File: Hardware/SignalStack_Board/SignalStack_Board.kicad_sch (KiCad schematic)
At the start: 66 parts, among them J1 Molex_uF_SV_06, J2 RJ45_LED_Shielded, J3 Molex_uF_SV_06, Q1 SI4156DY, Q2 SI4156DY, Q3 SI4156DY, Q4 SI4156DY, Q5 SI4156DY, Q6 SI4156DY, Q7 SI4156DY, Q8 SI4156DY, U1 OKI, U10 74LVC2G04, U2 SMAJ12CA, U3 Teensy4.1_DEV-16771, U4 TSR_1-2450, U5 IRS2005S, U6 IRS2005S, U7 74LVC2G04, U8 IRS2005S, U9 IRS2005S

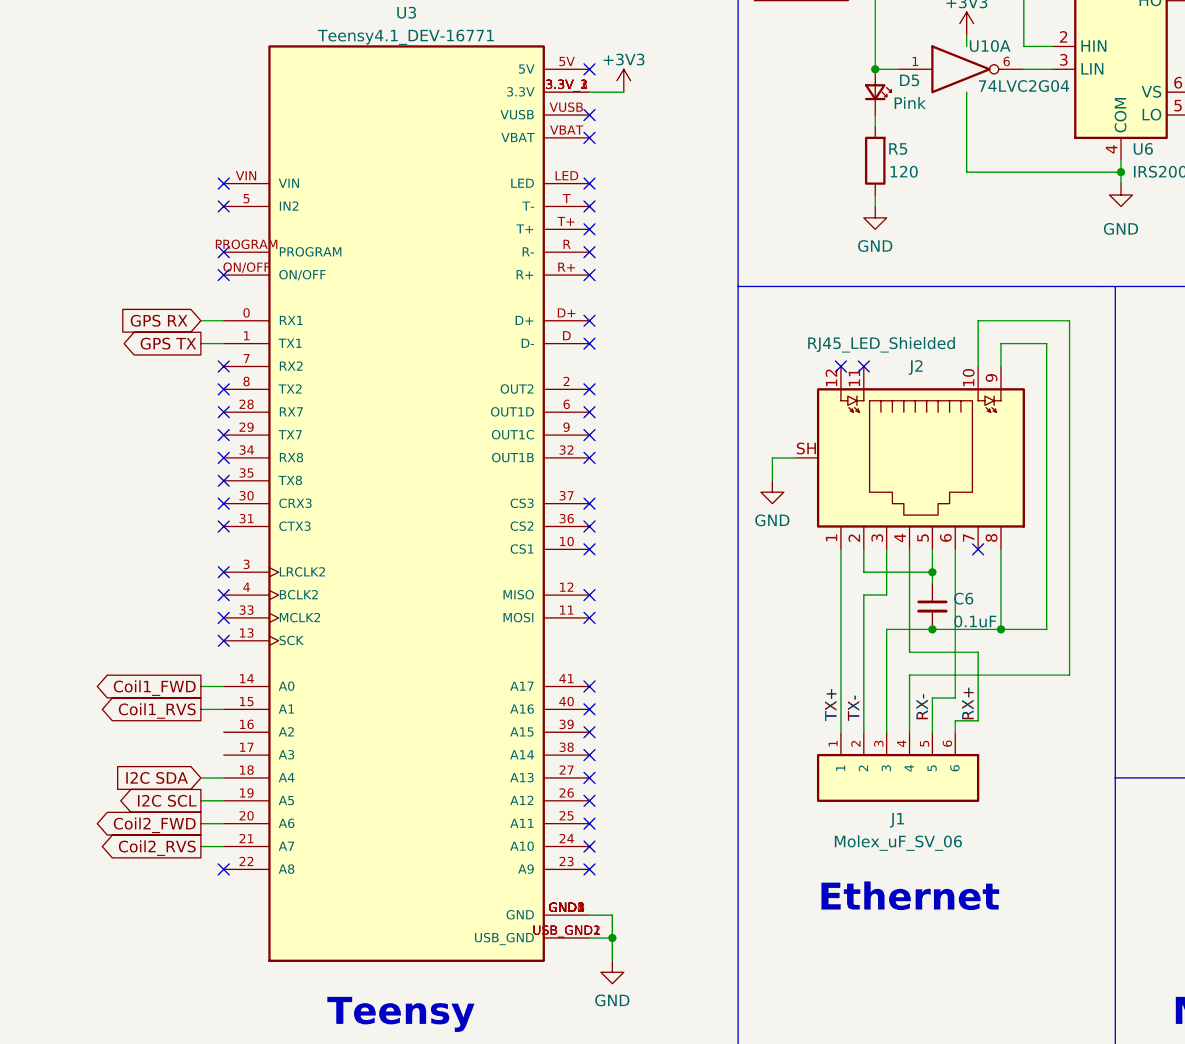
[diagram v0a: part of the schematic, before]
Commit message: Began Rev2 work
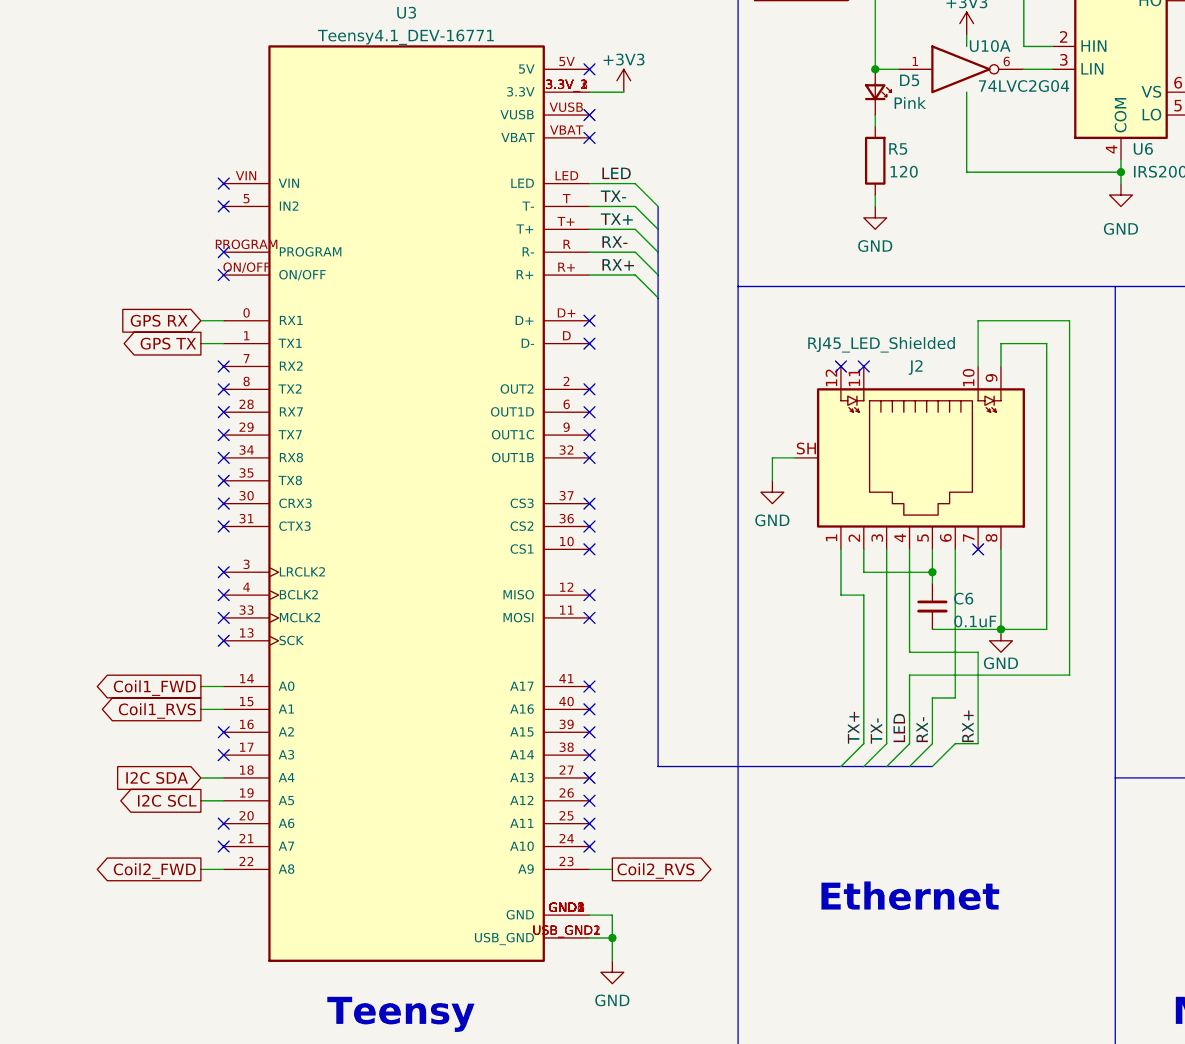
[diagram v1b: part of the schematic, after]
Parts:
- removed J1: Molex_uF_SV_06, Connector_PinHeader_2.00mm:PinHeader_2x03_P2.00mm_Vertical, symbol MRDT_Connectors:Molex_uF_SV_06
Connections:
- net Coil2_FWD: now also U3.22 (A8); no longer U3.20 (A6)
- net Coil2_RVS: now also U3.23 (A9); no longer U3.21 (A7)
- net GND: now also C6.2, J2.8, J2.9
- net RX+: now also U3.R+
- net RX-: now also U3.R (R-)
- net TX+: now also U3.T+
- net TX-: now also U3.T (T-)
- net LED: now reaches U3.LED
- net LED: now also J2.10
- no-connect marks 48 -> 45

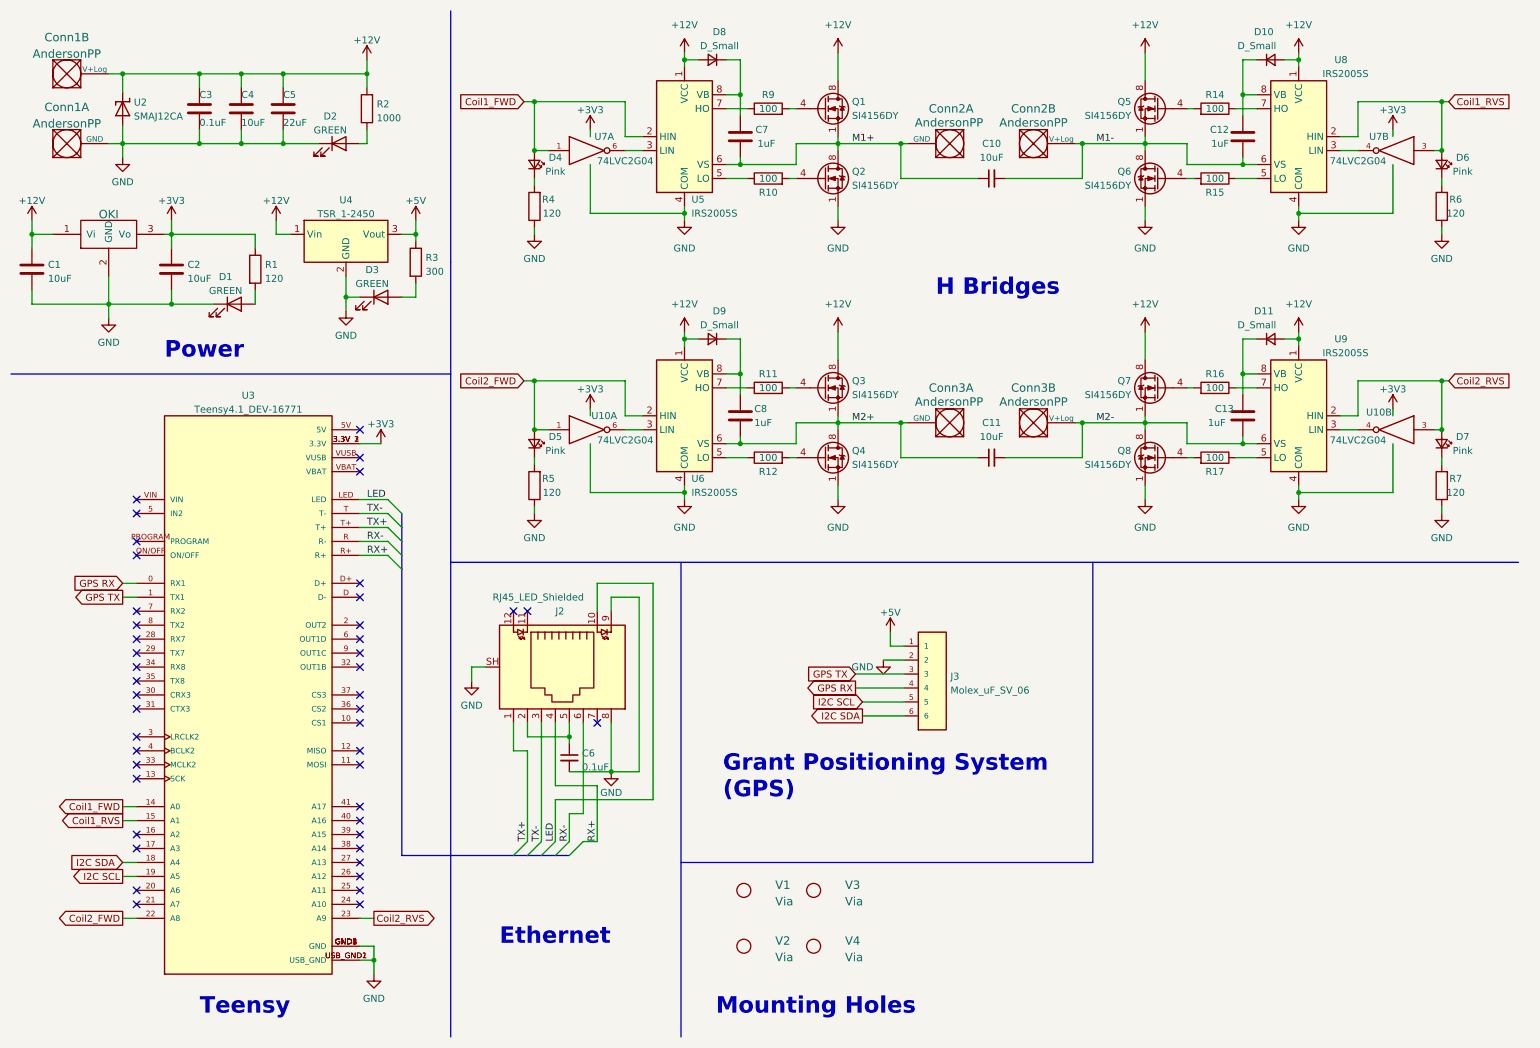
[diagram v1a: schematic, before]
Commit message: Updated schematic
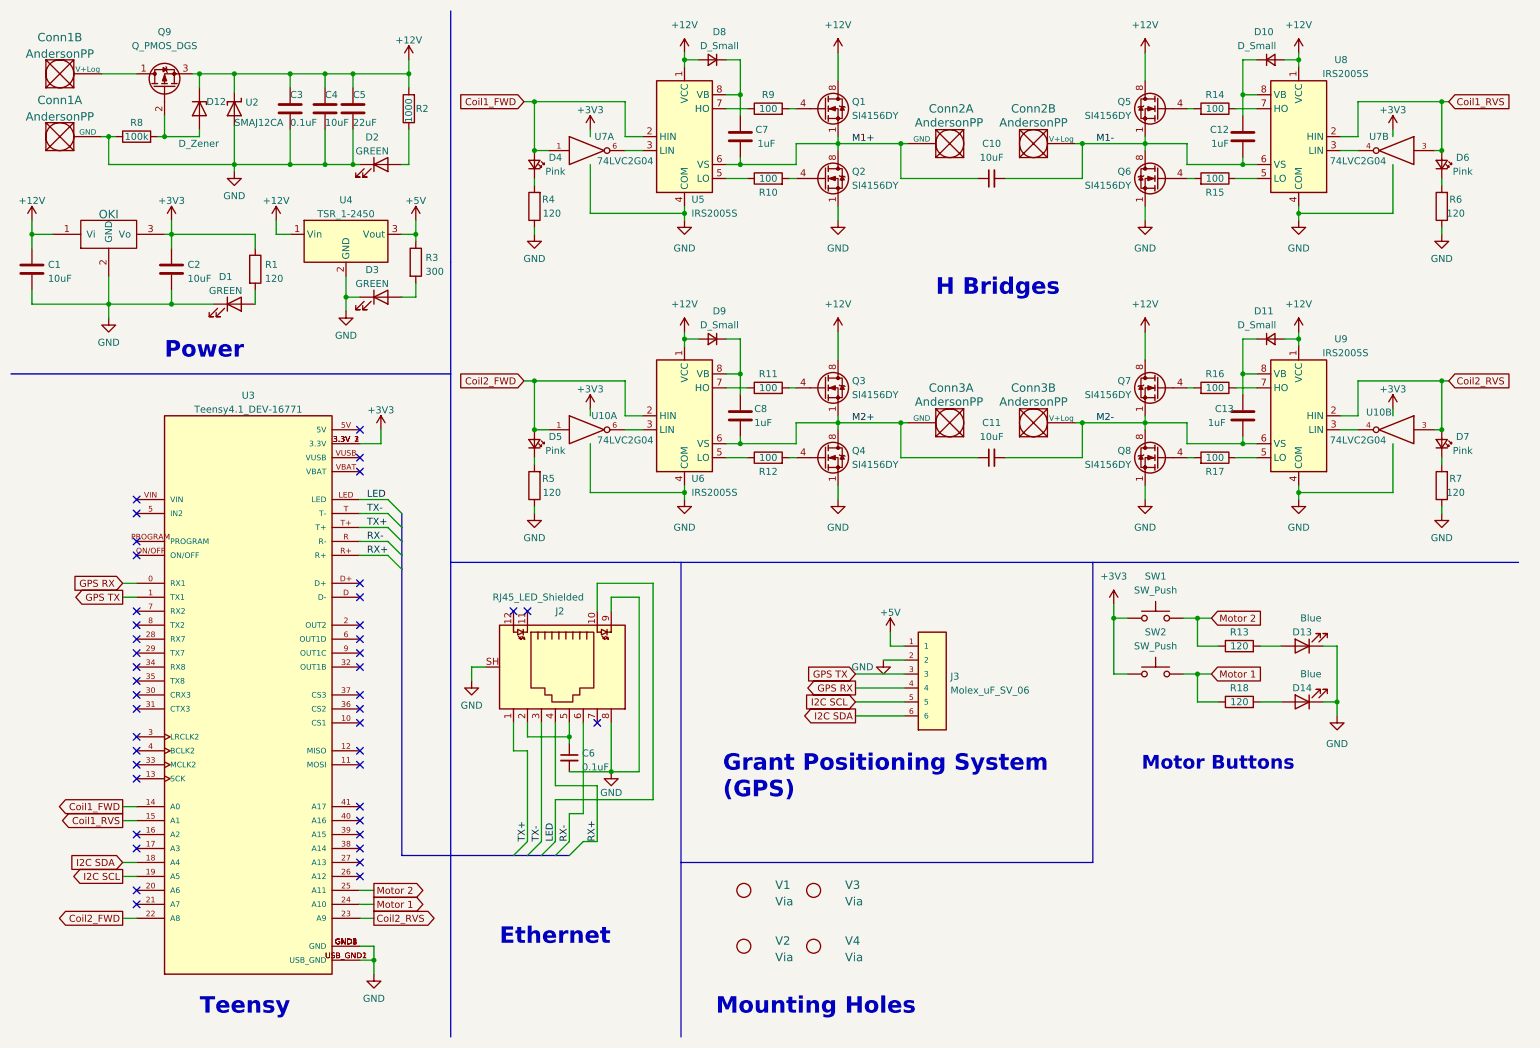
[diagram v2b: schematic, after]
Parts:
- added D12: D_Zener, Package_TO_SOT_SMD:SOT-23-3, symbol Device:D_Zener
- added D13, D14: Blue, LED_SMD:LED_0603_1608Metric_Pad1.05x0.95mm_HandSolder, symbol Device:LED
- added Q9: Q_PMOS_DGS, Package_TO_SOT_SMD:TO-252-3_TabPin2, symbol Device:Q_PMOS_DGS
- added R13, R18: 120, Resistor_SMD:R_0603_1608Metric_Pad0.98x0.95mm_HandSolder, symbol Device:R
- added R8: 100k, Resistor_SMD:R_0603_1608Metric_Pad0.98x0.95mm_HandSolder, symbol Device:R
- added SW1, SW2: SW_Push, Button_Switch_SMD:SW_SPST_TL3305A, symbol Switch:SW_Push
- J3: footprint MRDT_Connectors:MOLEX_uF_S_06_Vertical -> Connector_Molex:Molex_SL_171971-0006_1x06_P2.54mm_Vertical
- U3: footprint MRDT_Shields:Teensy_4_1_Bare -> MRDT_Shields:Teensy_4_1_Ethernet
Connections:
- net +12V: now also D12.1 (K), Q9.3 (S); no longer Conn1.2 (V+Log)
- net +3V3: now also SW1.1, SW2.1
- net GND: now also D13.1 (K), D14.1 (K), R8.1
- net Motor 1: now reaches U3.24 (A10)
- net Motor 1: now also R18.1, SW2.2
- net Motor 2: now reaches U3.25 (A11)
- net Motor 2: now also R13.1, SW1.2
- new net: D13.2 (A), R13.2
- new net: Conn1.2 (V+Log), Q9.1 (D)
- new net: D12.2 (A), Q9.2 (G), R8.2
- new net: D14.2 (A), R18.2
- no-connect marks 45 -> 43
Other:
- note added: "Motor Buttons"
- moved on the sheet: C3, C4, C5, Conn1A, Conn1B, D2, R2, U2
